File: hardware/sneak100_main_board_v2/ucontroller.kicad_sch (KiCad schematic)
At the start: 26 parts, among them SW1 SW_Push, U1 STM32F405RGTx, Y1 8MHz

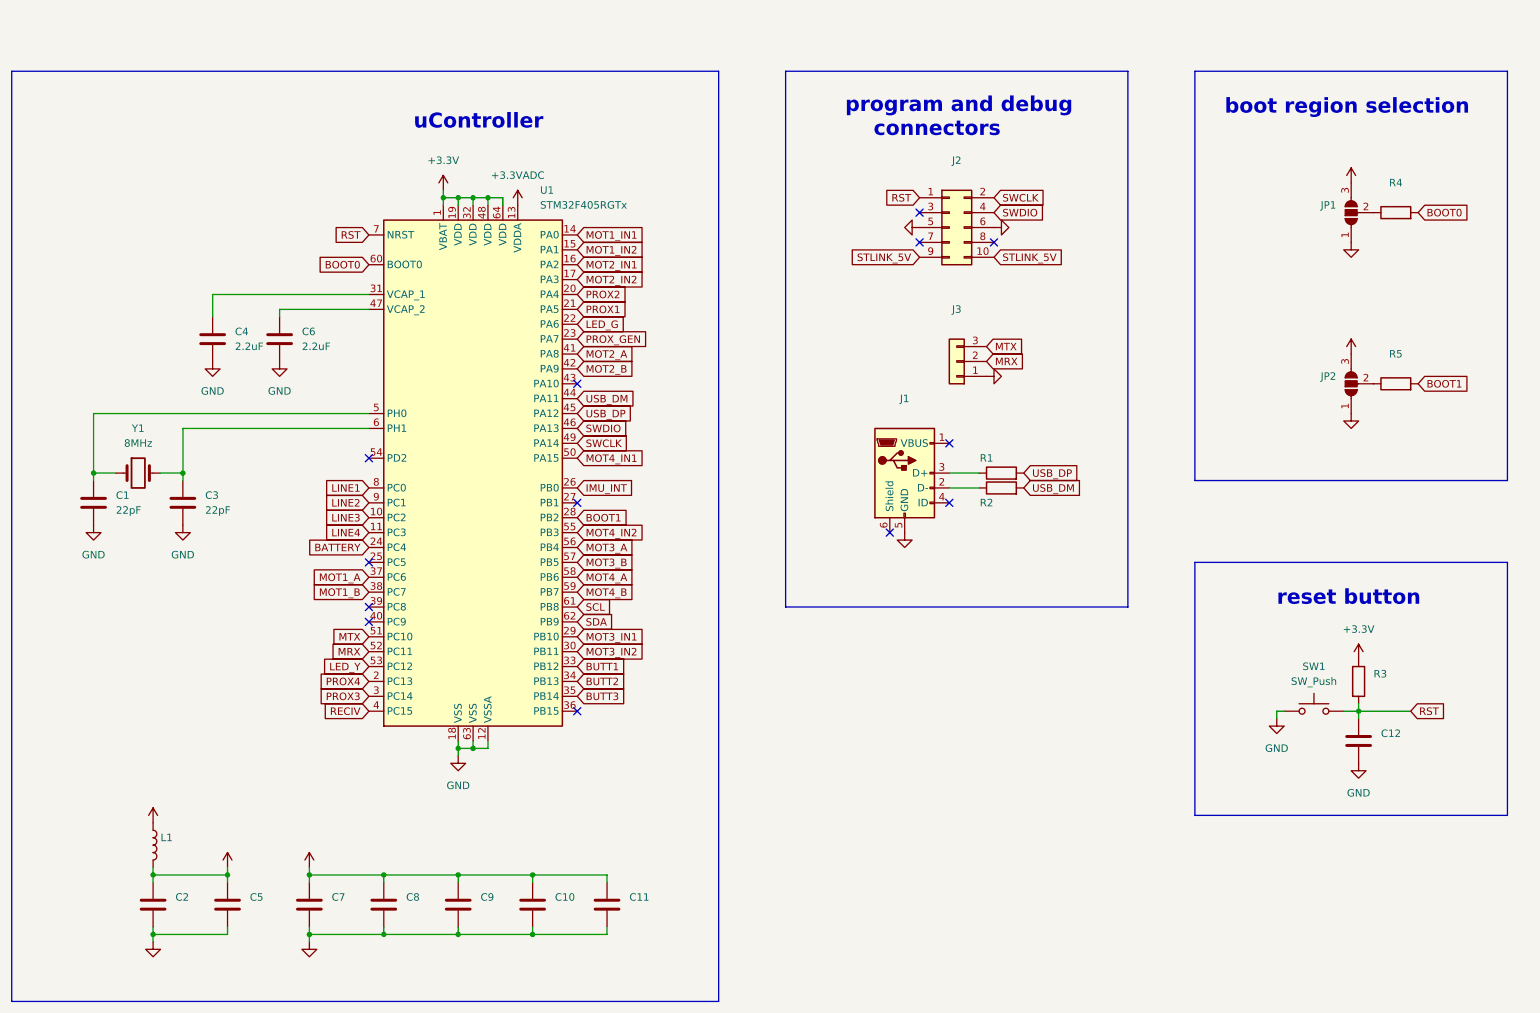
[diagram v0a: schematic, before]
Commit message: PCB version 2.0 schematic progress
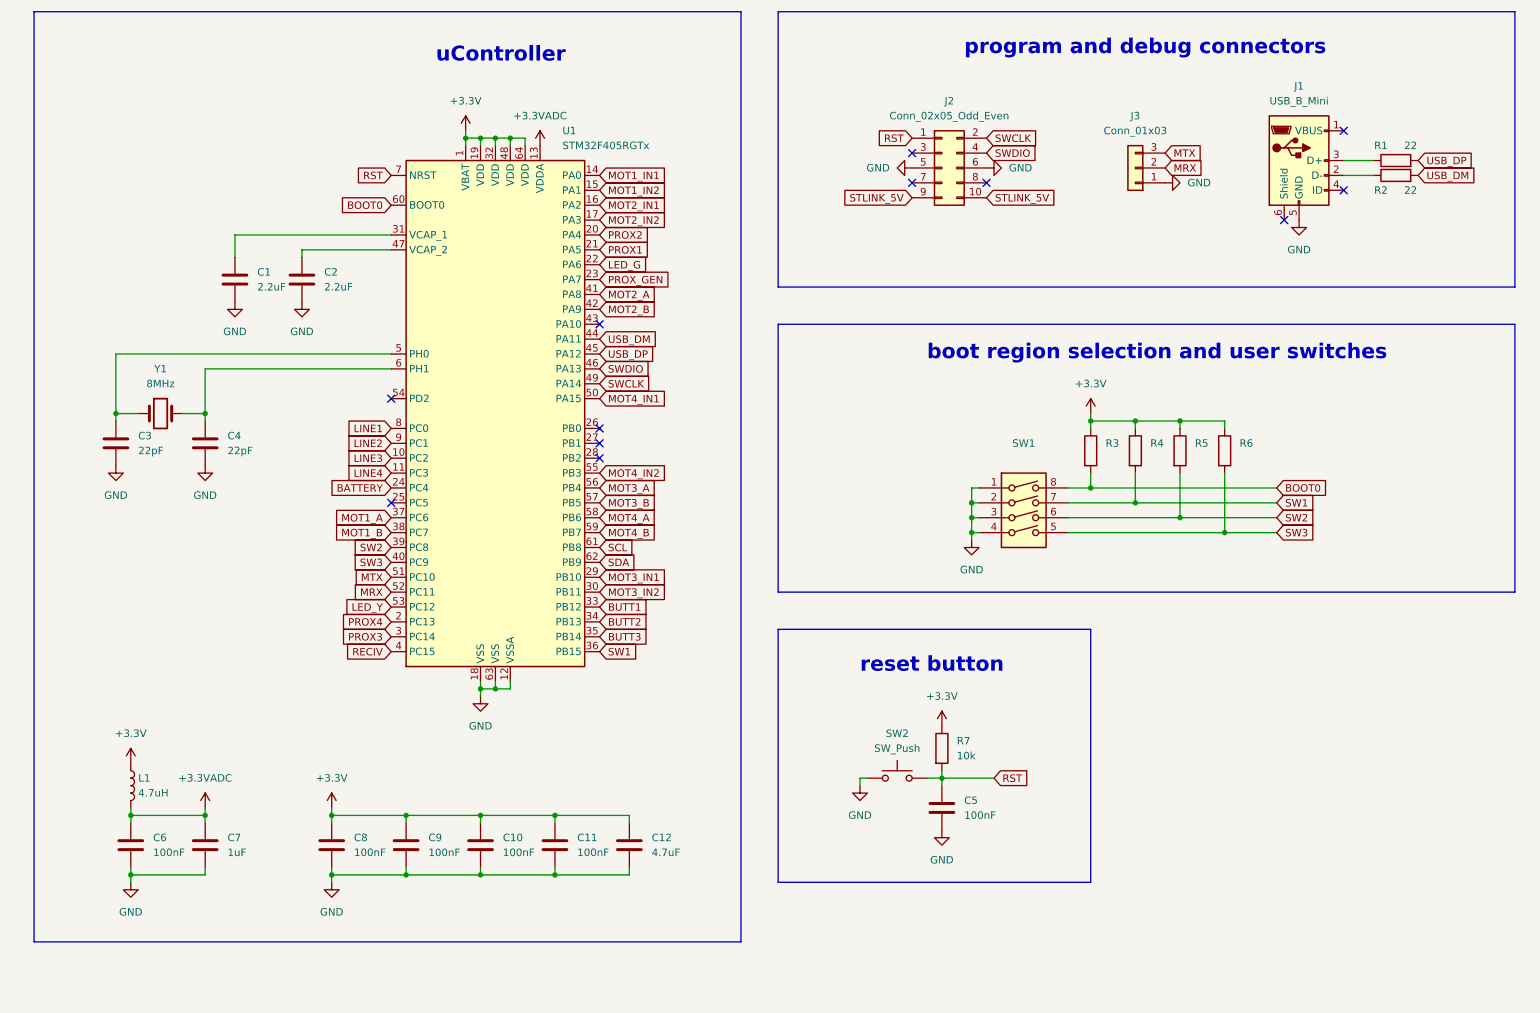
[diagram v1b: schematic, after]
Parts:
- removed JP1, JP2: (no value), symbol Jumper:SolderJumper_3_Open
- added R3, R6: (no value), symbol Device:R
- added SW1: (no value), symbol Switch:SW_DIP_x04
- C10: renamed from C9; value (none) -> 100nF
- C11: renamed from C10; value (none) -> 100nF
- C12: renamed from C11; value (none) -> 4.7uF
- C5: renamed from C12; value (none) -> 100nF
- C6: renamed from C2; value (none) -> 100nF
- C7: renamed from C5; value (none) -> 1uF
- C8: renamed from C7; value (none) -> 100nF
- C9: renamed from C8; value (none) -> 100nF
- J1: value (none) -> USB_B_Mini
- J2: value (none) -> Conn_02x05_Odd_Even
- J3: value (none) -> Conn_01x03
- L1: value (none) -> 4.7uH
- R1, R2: value (none) -> 22
- R7: renamed from R3; value (none) -> 10k
- renumbered C4 to C1, C6 to C2, C1 to C3, C3 to C4, SW1 to SW2
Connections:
- net +3V3: now also R4.1, R5.1, R3.1, R6.1
- net BOOT0: now also R3.2, SW1.8; no longer R4.2
- net GND: now also SW1.1, SW1.2, SW1.3, SW1.4
- net SW1: now reaches U1.36 (PB15)
- net SW1: now also R4.2, SW1.7
- net SW2: now reaches U1.39 (PC8)
- net SW2: now also R5.2, SW1.6
- net SW3: now reaches U1.40 (PC9)
- net SW3: now also R6.2, SW1.5
- net BOOT1: no longer names the net of U1.28 (PB2)
- net BOOT1: no longer R5.2
- net IMU_INT: no longer names the net of U1.26 (PB0)
- no-connect marks 13 -> 12
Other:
- note added: "boot region selection and user switches"
- note removed: "boot region selection"
- moved on the sheet: C1, C10, C11, C12, C2, C3, C4, C5, C6, C7, C8, C9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
